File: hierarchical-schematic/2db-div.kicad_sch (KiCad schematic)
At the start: 28 parts, among them J1001 Conn_01x02, J1002 From R2, J1003 Conn_01x02, J1004 Out, SW1001 2dB, SW1002 Video, U1001 MC1458, U1002 MC1458

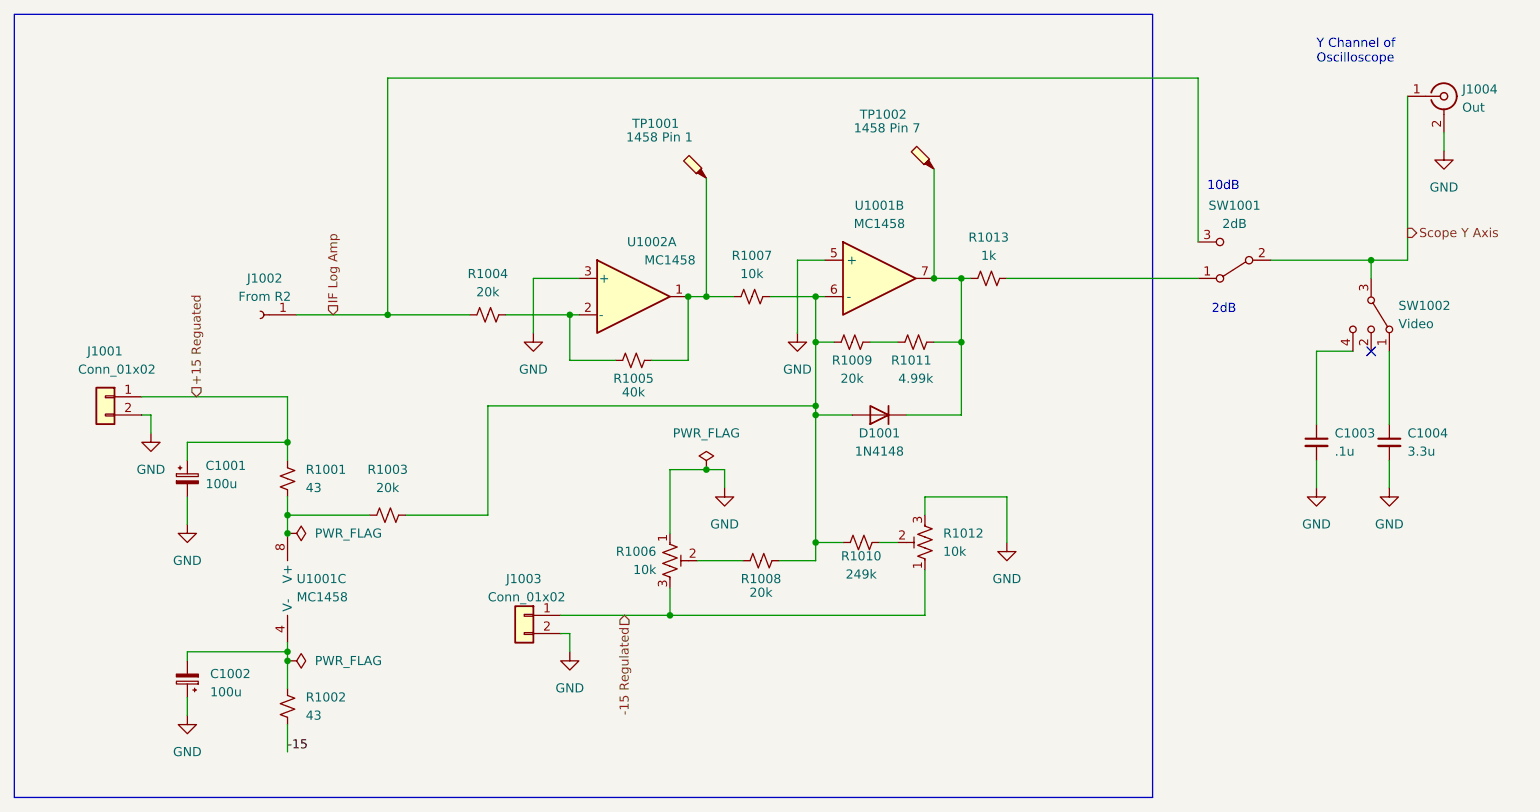
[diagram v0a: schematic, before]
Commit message: hierarchical schematic updated to pass erc
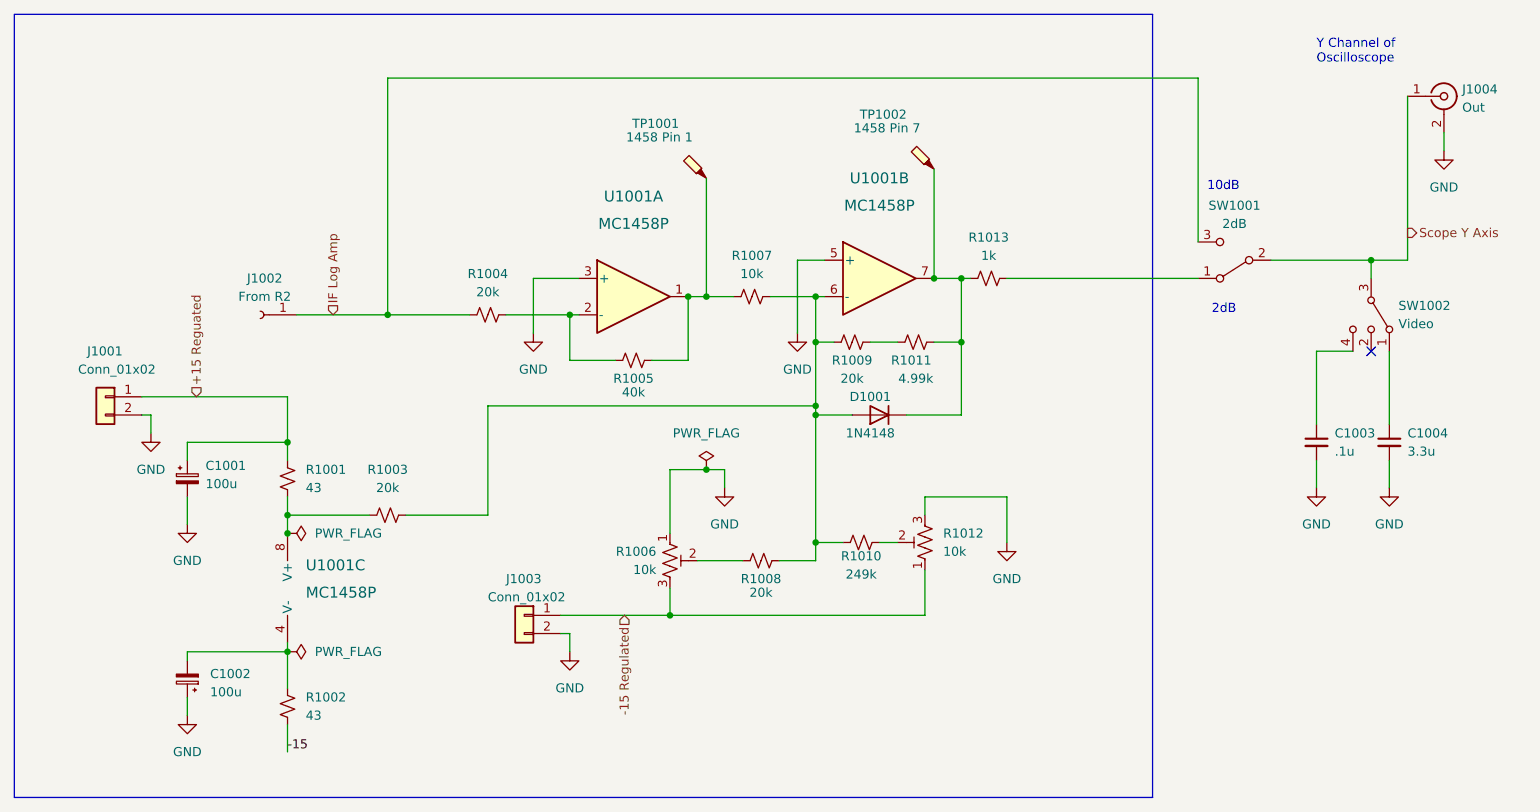
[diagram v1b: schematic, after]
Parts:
- removed U1001: MC1458, 2db-div:MC1458P, symbol Device:Opamp_Dual
- removed U1002: MC1458, 2db-div:MC1458P, symbol 2db-div:MC1458P
- added U1001: MC1458P, symbol spectrum analyzer:MC1458P
- D1001: symbol 2db-div:1N4152 -> Diode:1N4152
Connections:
- net GND: now also U1001.3 (+), U1001.5 (+)
- net at D1001.2 (A), R1003.1, R1007.2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: now also U1001.6 (-)
- net at D1001.1 (K), R1011.2, R1013.1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: now also U1001.7
- net at R1005.2, R1007.1, TP1001.1: now also U1001.1
- net at R1001.1, R1003.2: now also U1001.8 (V+)
- net at C1002.2, R1002.2: now also U1001.4 (V-)
- net at R1004.2, R1005.1: now also U1001.2 (-)

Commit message: v7 conversion
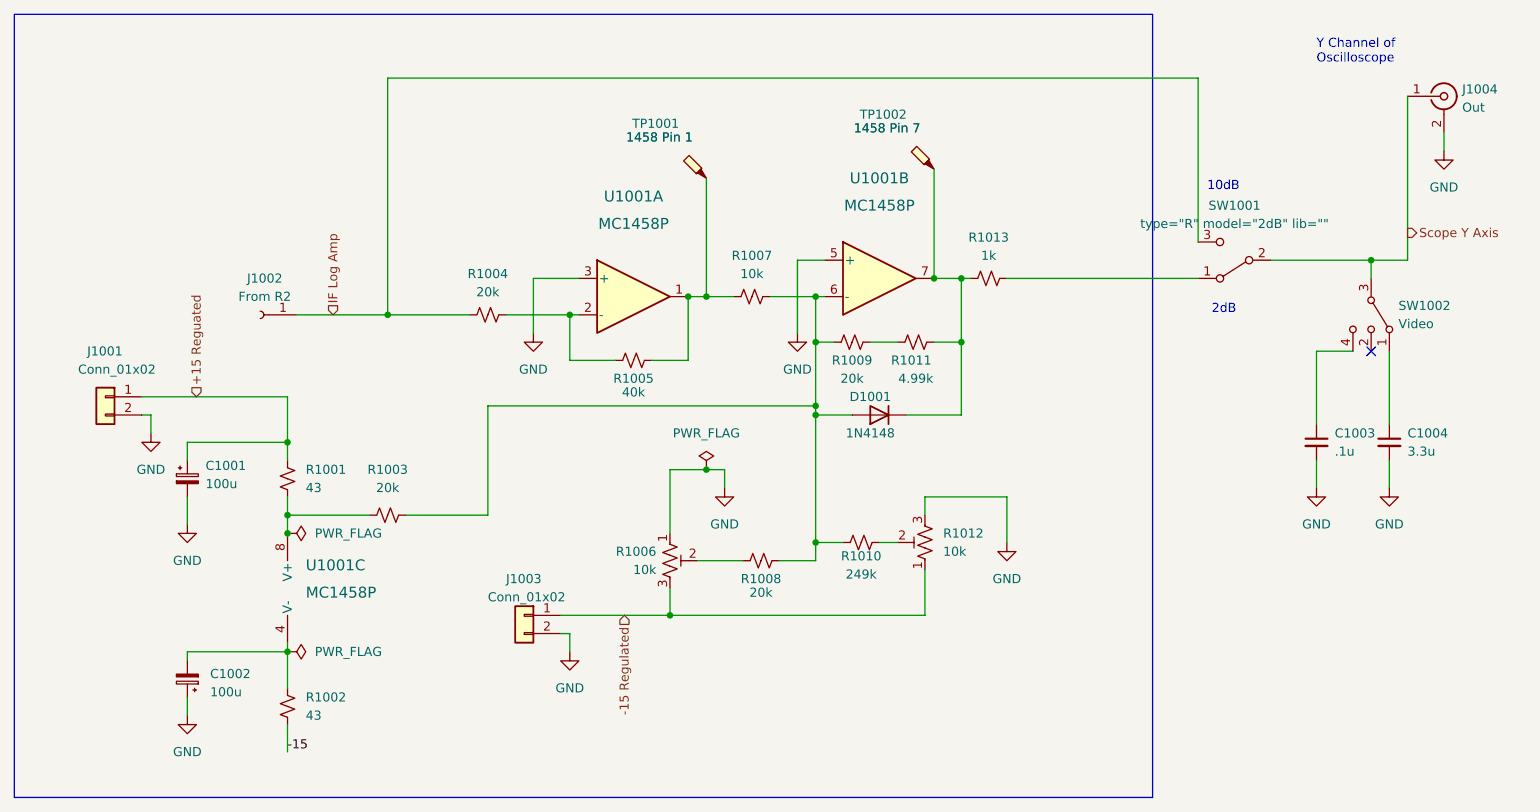
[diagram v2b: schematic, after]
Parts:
- D1001: Spice_Lib_File 2db-div-spice\fairch.lib -> (none); Spice_Model 1N4152 -> (none); Spice_Netlist_Enabled Y -> (none); Spice_Node_Sequence 2 1 -> (none); Spice_Primitive D -> (none)
- J1001, J1003: Spice_Model Conn_01x02 -> (none); Spice_Netlist_Enabled N -> (none); Spice_Primitive J -> (none)
- J1004: Spice_Model Conn_Coaxial -> (none); Spice_Netlist_Enabled N -> (none); Spice_Primitive J -> (none)
- R1006: Spice_Lib_File 2db-div-spice\Pot.lib -> (none); Spice_Model pot_lin -> (none); Spice_Netlist_Enabled Y -> (none); Spice_Primitive X -> (none)
- R1012: Spice_Lib_File 2db-div-spice\Pot2.lib -> (none); Spice_Model pot_lin2 -> (none); Spice_Netlist_Enabled Y -> (none); Spice_Primitive X -> (none)
- SW1001: value 2dB -> ${SIM.PARAMS}; Spice_Netlist_Enabled N -> (none); Spice_Primitive R -> (none)
- TP1001: value 1458 Pin 1 -> ${SIM.PARAMS}; Spice_Netlist_Enabled N -> (none)
- TP1002: value 1458 Pin 7 -> ${SIM.PARAMS}; Spice_Netlist_Enabled N -> (none)
